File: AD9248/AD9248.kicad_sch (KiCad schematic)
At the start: 14 parts, among them J1 Conn_01x01_Pin, J2 Conn_01x01_Pin, U1 TLV70018DCKR, U2 AD9284BCPZ-250, U3 TLV70018DCKR

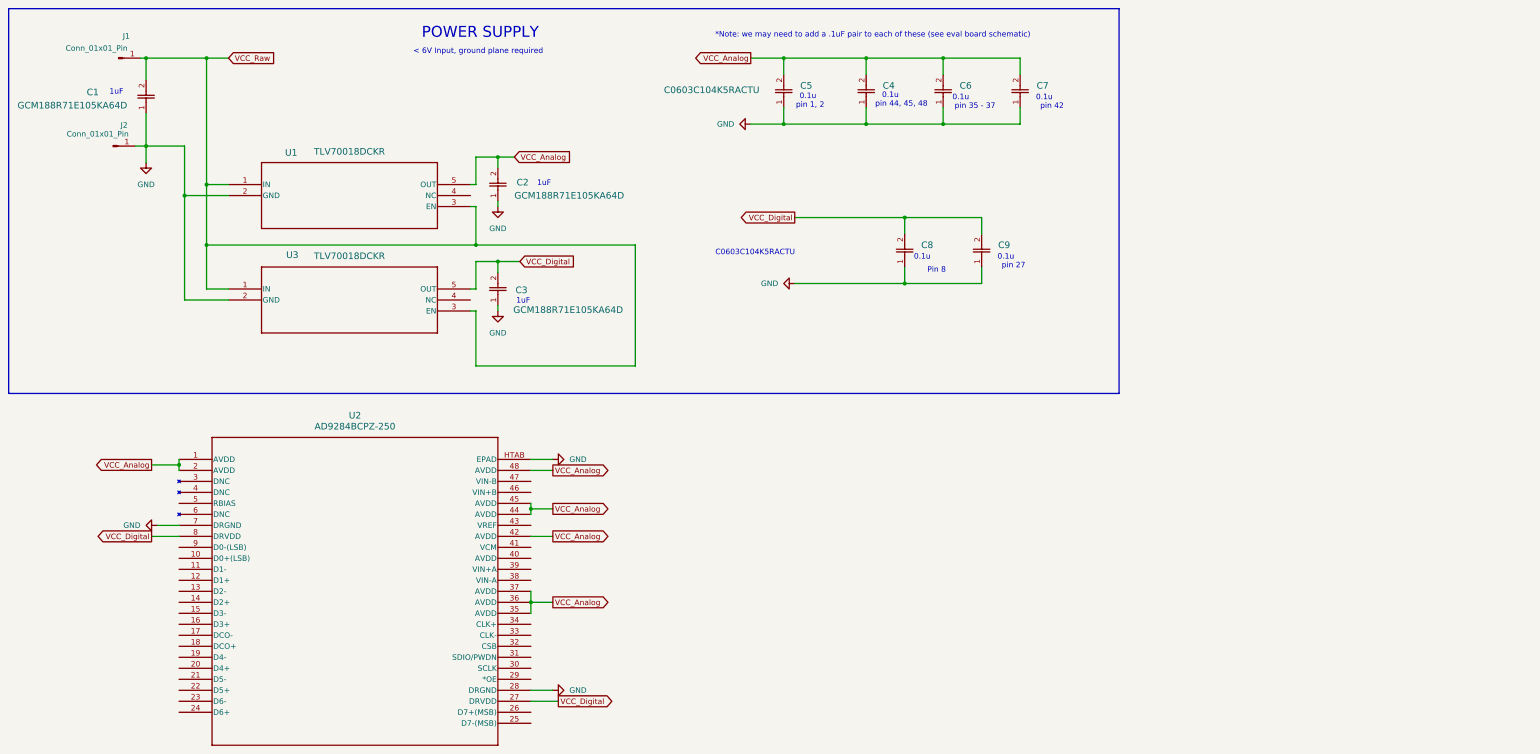
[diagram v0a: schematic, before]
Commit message: Schematic for ADC breakout complete (ish)
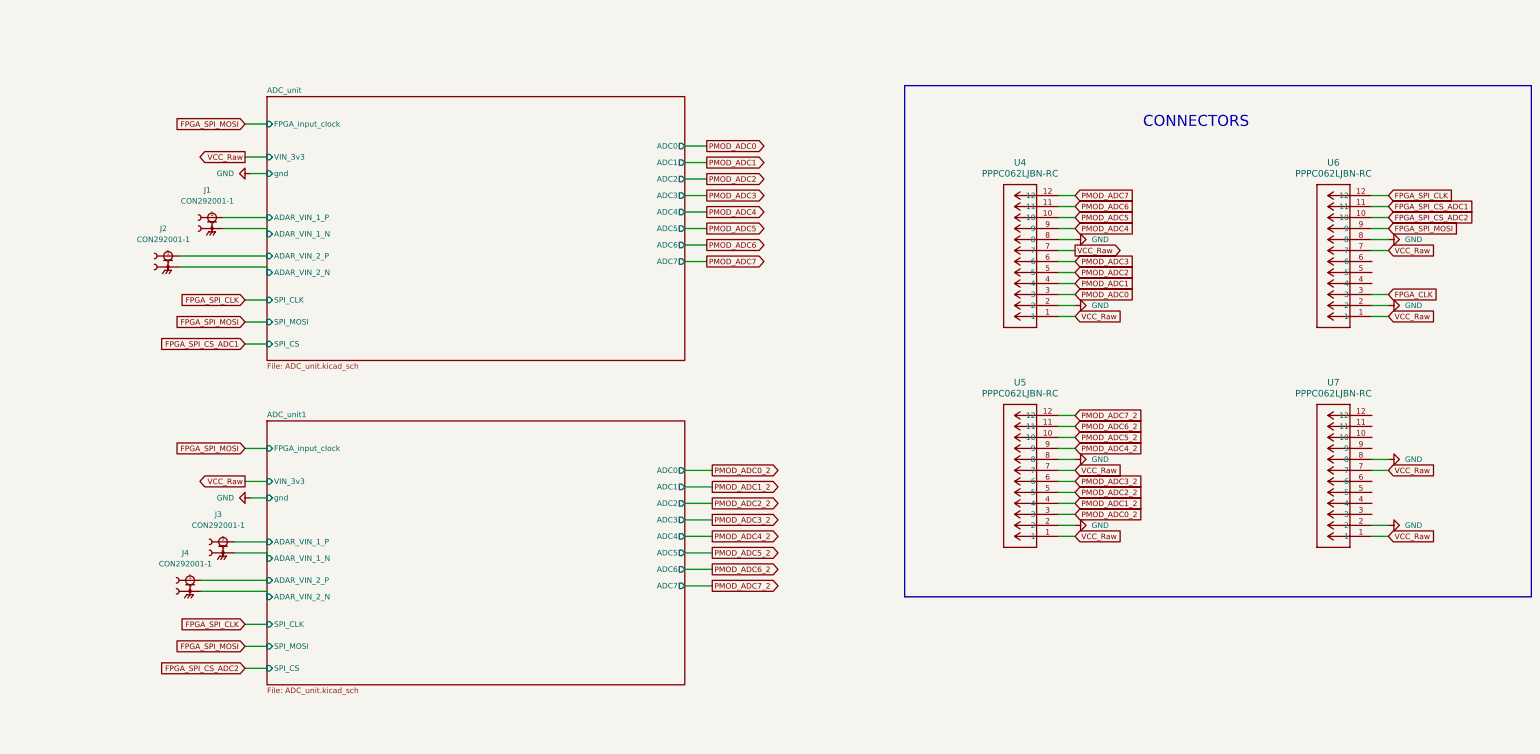
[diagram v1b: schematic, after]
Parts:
- removed C1, C2, C3: GCM188R71E105KA64D, part_library:GCM188R71E105KA64D, symbol GCM188R71E105KA64D:GCM188R71E105KA64D
- removed C4, C5, C6, C7, C8, C9: C0603C104K5RACTU, part_library:C0603C104K5RACTU, symbol C0603C104K5RACTU:C0603C104K5RACTU
- removed J1, J2: Conn_01x01_Pin, symbol Connector:Conn_01x01_Pin
- removed U1, U3: TLV70018DCKR, part_library:TLV70018DCKR, symbol TLV70018DCKR:TLV70018DCKR
- removed U2: AD9284BCPZ-250, part_library:AD9284, symbol AD9248:AD9284BCPZ-250
- added J1, J2, J3, J4: CON292001-1, part_library:TE_CON292001-1, symbol CON292001-1:CON292001-1
- added U4, U5, U6, U7: PPPC062LJBN-RC, part_library:CONN_PPPC062LJBN-RC_SUL, symbol PPPC062LJBN_RC:PPPC062LJBN-RC
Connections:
- net GND: now also U4.2, U4.8, U5.2, U5.8, U6.2, U6.8, U7.2, U7.8
- net VCC_Raw: now also U4.1, U4.7, U5.1, U5.7, U6.1, U6.7, U7.1, U7.7
- new net ADC_unit/ADAR_VIN_1_N: J1.2, J1.3, J1.4
- new net ADC_unit/ADAR_VIN_1_P: J1.1
- new net ADC_unit/ADAR_VIN_2_N: J2.2, J2.3, J2.4
- new net ADC_unit/ADAR_VIN_2_P: J2.1
- new net ADC_unit1/ADAR_VIN_1_N: J3.2, J3.3, J3.4
- new net ADC_unit1/ADAR_VIN_1_P: J3.1
- new net ADC_unit1/ADAR_VIN_2_N: J4.2, J4.3, J4.4
- new net ADC_unit1/ADAR_VIN_2_P: J4.1
- new net FPGA_CLK: U6.3
- new net FPGA_SPI_CLK: U6.12
- new net FPGA_SPI_CS_ADC1: U6.11
- new net FPGA_SPI_CS_ADC2: U6.10
- new net FPGA_SPI_MOSI: U6.9
- new net PMOD_ADC0: U4.3
- new net PMOD_ADC0_2: U5.3
- new net PMOD_ADC1: U4.4
- new net PMOD_ADC1_2: U5.4
- new net PMOD_ADC2: U4.5
- new net PMOD_ADC2_2: U5.5
- new net PMOD_ADC3: U4.6
- new net PMOD_ADC3_2: U5.6
- new net PMOD_ADC4: U4.9
- new net PMOD_ADC4_2: U5.9
- new net PMOD_ADC5: U4.10
- new net PMOD_ADC5_2: U5.10
- new net PMOD_ADC6: U4.11
- new net PMOD_ADC6_2: U5.11
- new net PMOD_ADC7: U4.12
- new net PMOD_ADC7_2: U5.12
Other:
- added sheet ADC_unit (ADC_unit.kicad_sch)
- added sheet ADC_unit1 (ADC_unit.kicad_sch)
- note added: "CONNECTORS"
- note removed: "*Note: we may need to add a .1uF pair to each of these (see eval board schematic)"
- note removed: "0.1u"
- note removed: "1uF"
- note removed: "< 6V Input, ground plane required"
- note removed: "C0603C104K5RACTU"
- note removed: "POWER SUPPLY"
- note removed: "Pin 8"
- note removed: "pin 1, 2"
- note removed: "pin 27"
- note removed: "pin 35 - 37"
- note removed: "pin 42"
- note removed: "pin 44, 45, 48"
